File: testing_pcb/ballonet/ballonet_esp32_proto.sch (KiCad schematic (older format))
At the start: 14 parts, among them M1 Motor_DC, M2 Motor_DC, U1 DOIT-ESP32-DEVKIT-V1-30, U2 GY-291-ADXL345-breakoout, U3 CJVL53L0XV2-VL53L0X-breakout, U4 Adafruit-BMP388-breakout, U5 Adafruit-DRV8833-breakout, U6 Polulu-S7V8F3-3V3

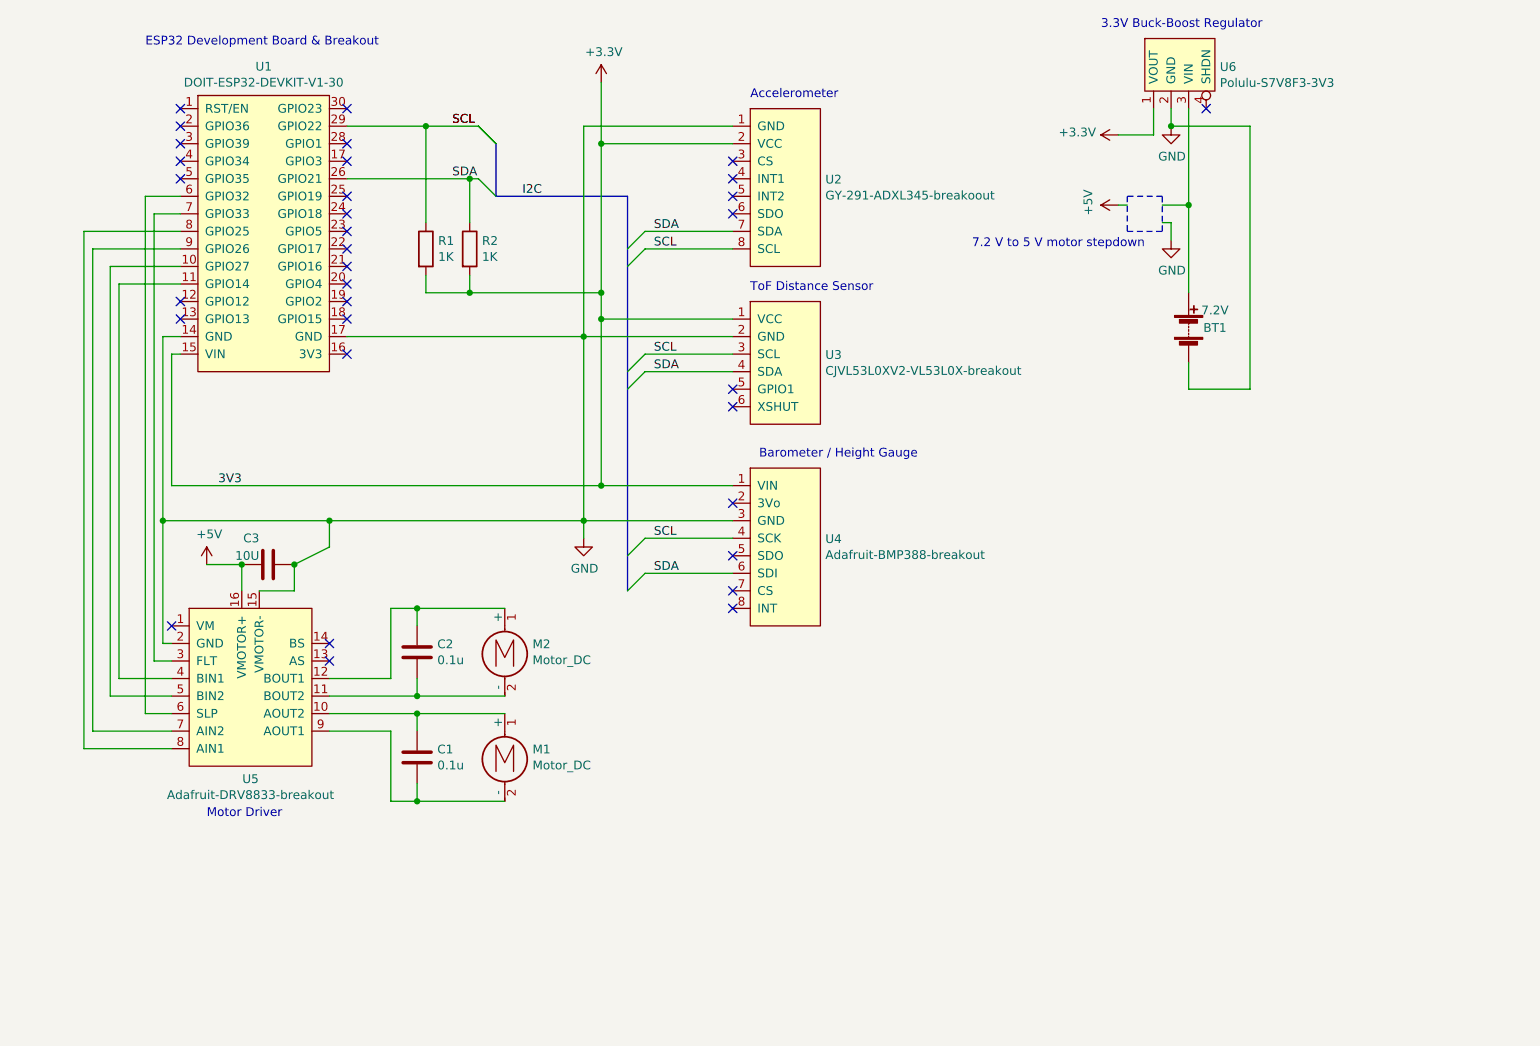
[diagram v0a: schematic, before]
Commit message: updated schematic
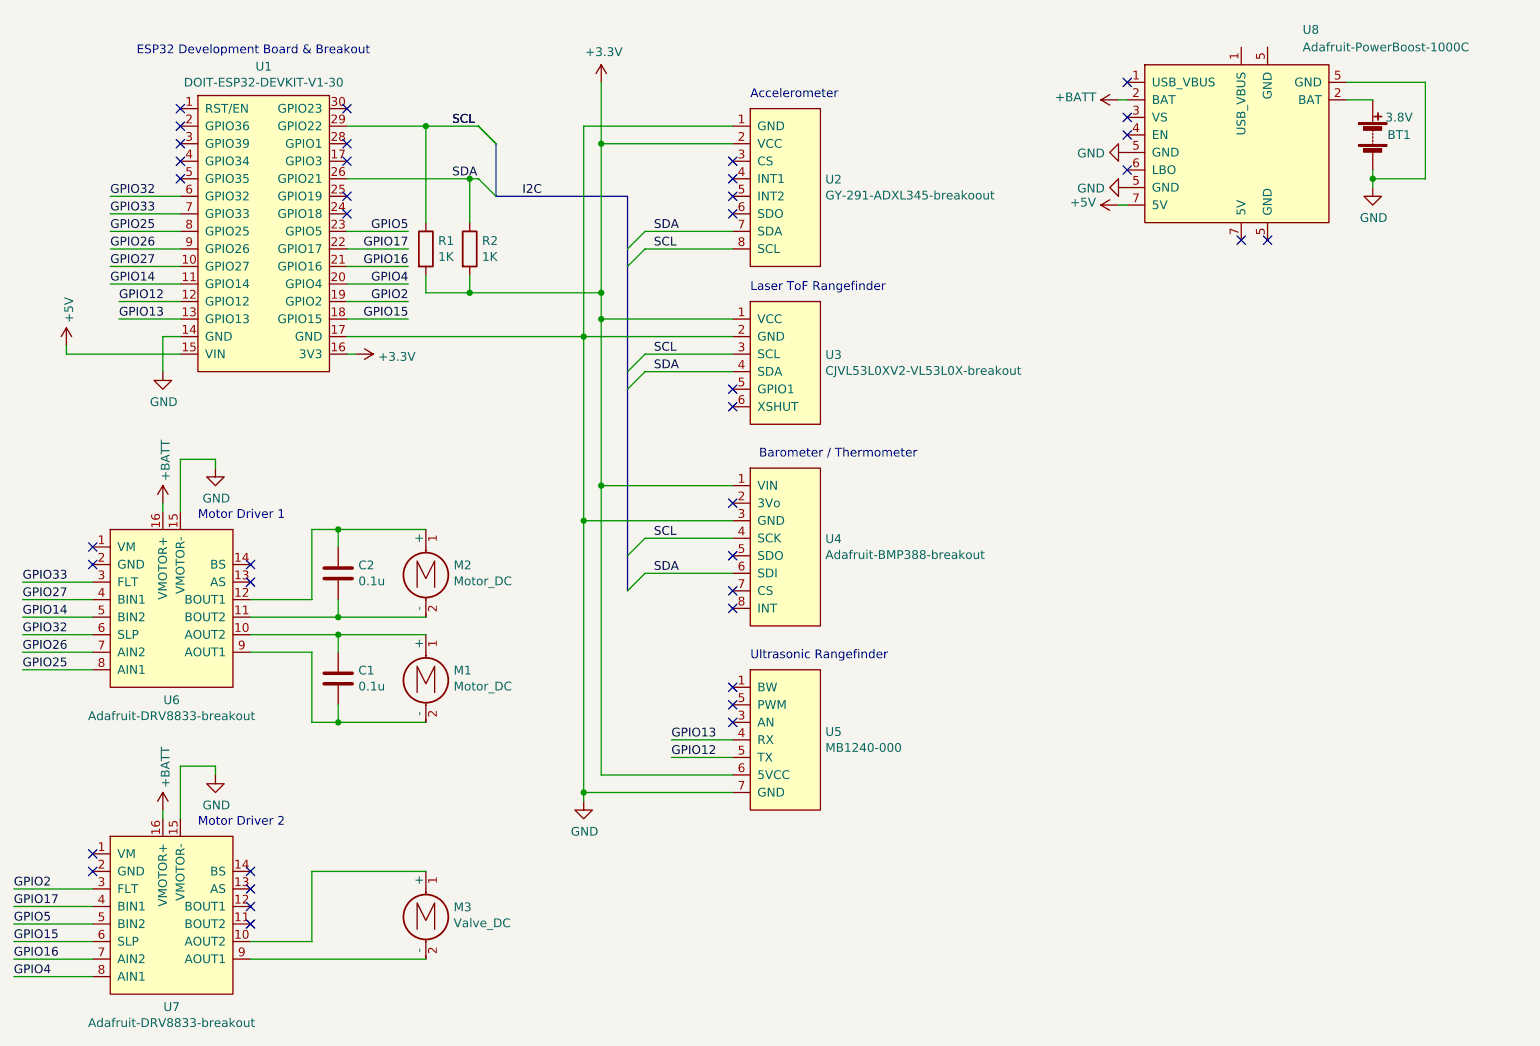
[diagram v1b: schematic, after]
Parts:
- removed C3: 10U, symbol Device:C
- removed U6: Polulu-S7V8F3-3V3, symbol adafruit-breakouts:Polulu-S7V8F3-3V3
- added M3: Valve_DC, symbol Motor:Motor_DC
- added U5: MB1240-000, symbol adafruit-breakouts:MB1240-000
- added U7: Adafruit-DRV8833-breakout, symbol adafruit-breakouts:Adafruit-DRV8833-breakout
- added U8: Adafruit-PowerBoost-1000C, symbol adafruit-breakouts:Adafruit-PowerBoost-1000C
- BT1: value 7.2V -> 3.8V
- renumbered U5 to U6
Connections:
- net labels added: +BATT, GPIO12, GPIO13, GPIO14, GPIO15, GPIO16, GPIO17, GPIO2, GPIO25, GPIO26, GPIO27, GPIO32, GPIO33, GPIO4, GPIO5
- net labels removed: 3V3
- wire segments 92 -> 103
- no-connect marks 33 -> 39
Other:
- note added: "Barometer / Thermometer\n"
- note added: "Laser ToF Rangefinder"
- note added: "Motor Driver 1\n"
- note added: "Motor Driver 2"
- note added: "Ultrasonic Rangefinder\n"
- note removed: "3.3V Buck-Boost Regulator"
- note removed: "7.2 V to 5 V motor stepdown"
- note removed: "Barometer / Height Gauge"
- note removed: "Motor Driver"
- note removed: "ToF Distance Sensor"
- moved on the sheet: BT1, C1, C2, M1, M2, U6
